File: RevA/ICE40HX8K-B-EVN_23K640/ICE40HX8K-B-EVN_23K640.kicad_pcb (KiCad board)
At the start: 2 copper layers, 19 parts, among them J1 2x20_Socket, U0 23K640, U1 23K640, U2 23K640, U3 23K640, U4 23K640, U5 23K640, U6 23K640, U7 23K640

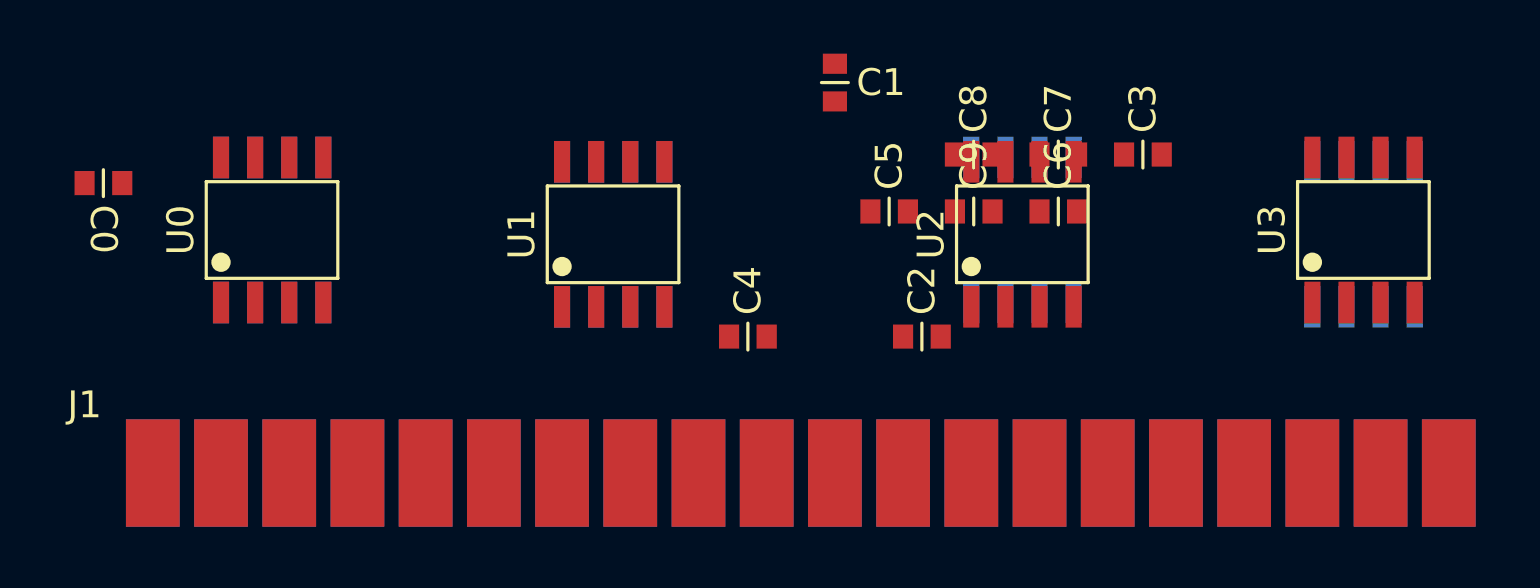
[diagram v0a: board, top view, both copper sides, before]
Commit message: routin
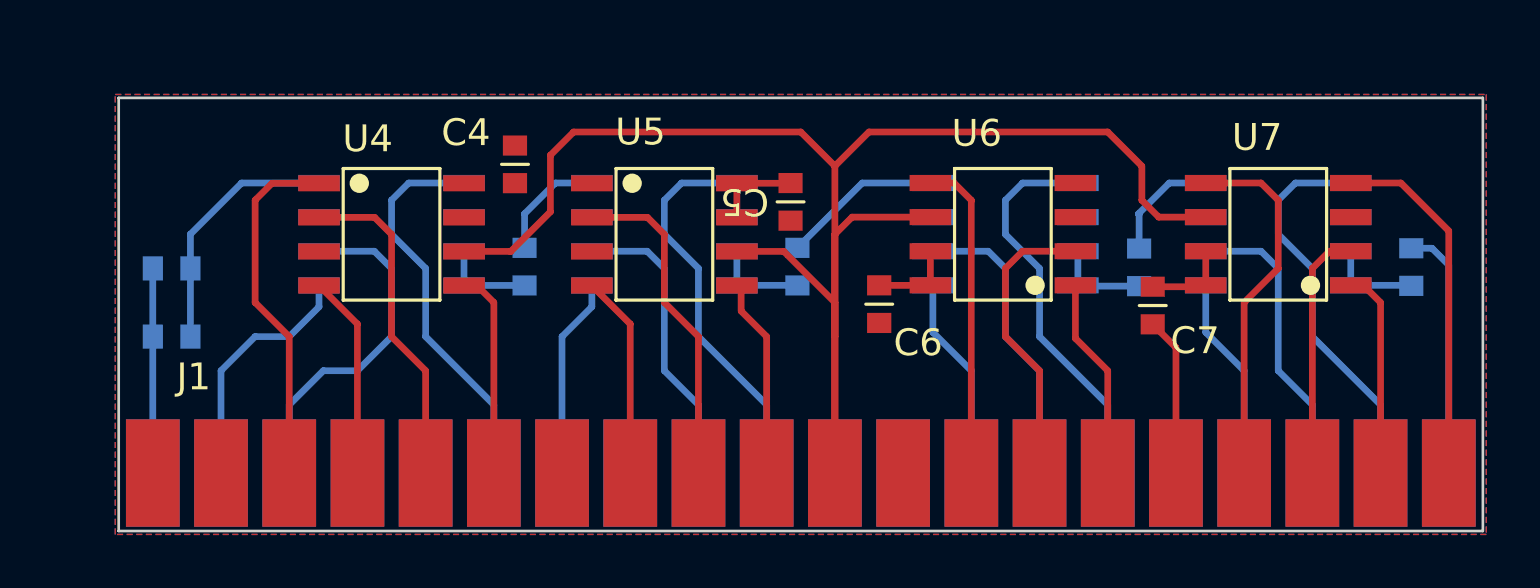
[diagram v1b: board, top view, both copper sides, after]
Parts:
- C0, C1, C2, C3, C8, C9, U0, U1, U2, U3: moved to B.Cu
- U4, U5, U6, U7: moved to F.Cu
- moved C9 28.8 mm to (67.4, 119.4), turned to 180 degrees
- moved C8 28.8 mm to (67.4, 116.8), turned to 180 degrees
- moved C0 15.2 mm to (79.9, 116.1), turned to -90 degrees
- moved C3 11.2 mm to (112.9, 116.1), turned to -90 degrees
- moved C4 10.7 mm to (79.5, 112.3), turned to -90 degrees
- moved C2 9.38 mm to (102.8, 116.1), turned to -90 degrees
- moved C7 7.60 mm to (103.3, 118.9), turned to 90 degrees
- moved C6 7.27 mm to (93.1, 118.9), turned to 90 degrees
- moved C1 7.00 mm to (90.0, 116.1)
- moved U5 5.33 mm to (82.4, 113.7), turned to -90 degrees
- moved U4 4.44 mm to (72.2, 113.7), turned to -90 degrees
- moved U3 4.02 mm to (105.2, 117.5), turned to 90 degrees
- moved U0 3.71 mm to (72.2, 117.5), turned to 90 degrees
- moved C5 2.99 mm to (89.8, 115.1), turned to 90 degrees
- moved U7 2.51 mm to (110.7, 117.5), turned to 90 degrees
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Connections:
- C7 pad 1: unconnected-(C7-Pad1) -> GND
- J1 pad 25: /nCS_6 -> /SI_6
- J1 pad 29: /SI_6 -> /nCS_6
- J1 pad 33: /nCS_7 -> /SI_7
- J1 pad 37: /SI_7 -> /nCS_7
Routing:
- net GND: track 0.00 -> 67.8 mm
- net Net-(J1-Pad21): track 0.00 -> 63.5 mm
- net +3V3: track 0.00 -> 31.5 mm
- net /SI_3: track 0.00 -> 14.7 mm
- net /SI_1: track 0.00 -> 14.7 mm
- net /SI_0: track 0.00 -> 14.7 mm
- net /SI_2: track 0.00 -> 14.7 mm
- net /SI_7: track 0.00 -> 13.7 mm
- net /nCS_4: track 0.00 -> 13.3 mm
- net /S0_0: track 0.00 -> 12.9 mm
- net /S0_4: track 0.00 -> 12.4 mm
- net /S0_5: track 0.00 -> 12.2 mm
- net /SI_6: track 0.00 -> 11.9 mm
- net /S0_3: track 0.00 -> 11.1 mm
- net /S0_1: track 0.00 -> 11.1 mm
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- added copper zone on B.Cu, net GND
- added copper zone on F.Cu, net GND
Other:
- board outline added: 50.8 x 16.1 mm
